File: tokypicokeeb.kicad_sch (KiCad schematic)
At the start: 119 parts, among them SW1 SW_Push, U1 PicoW

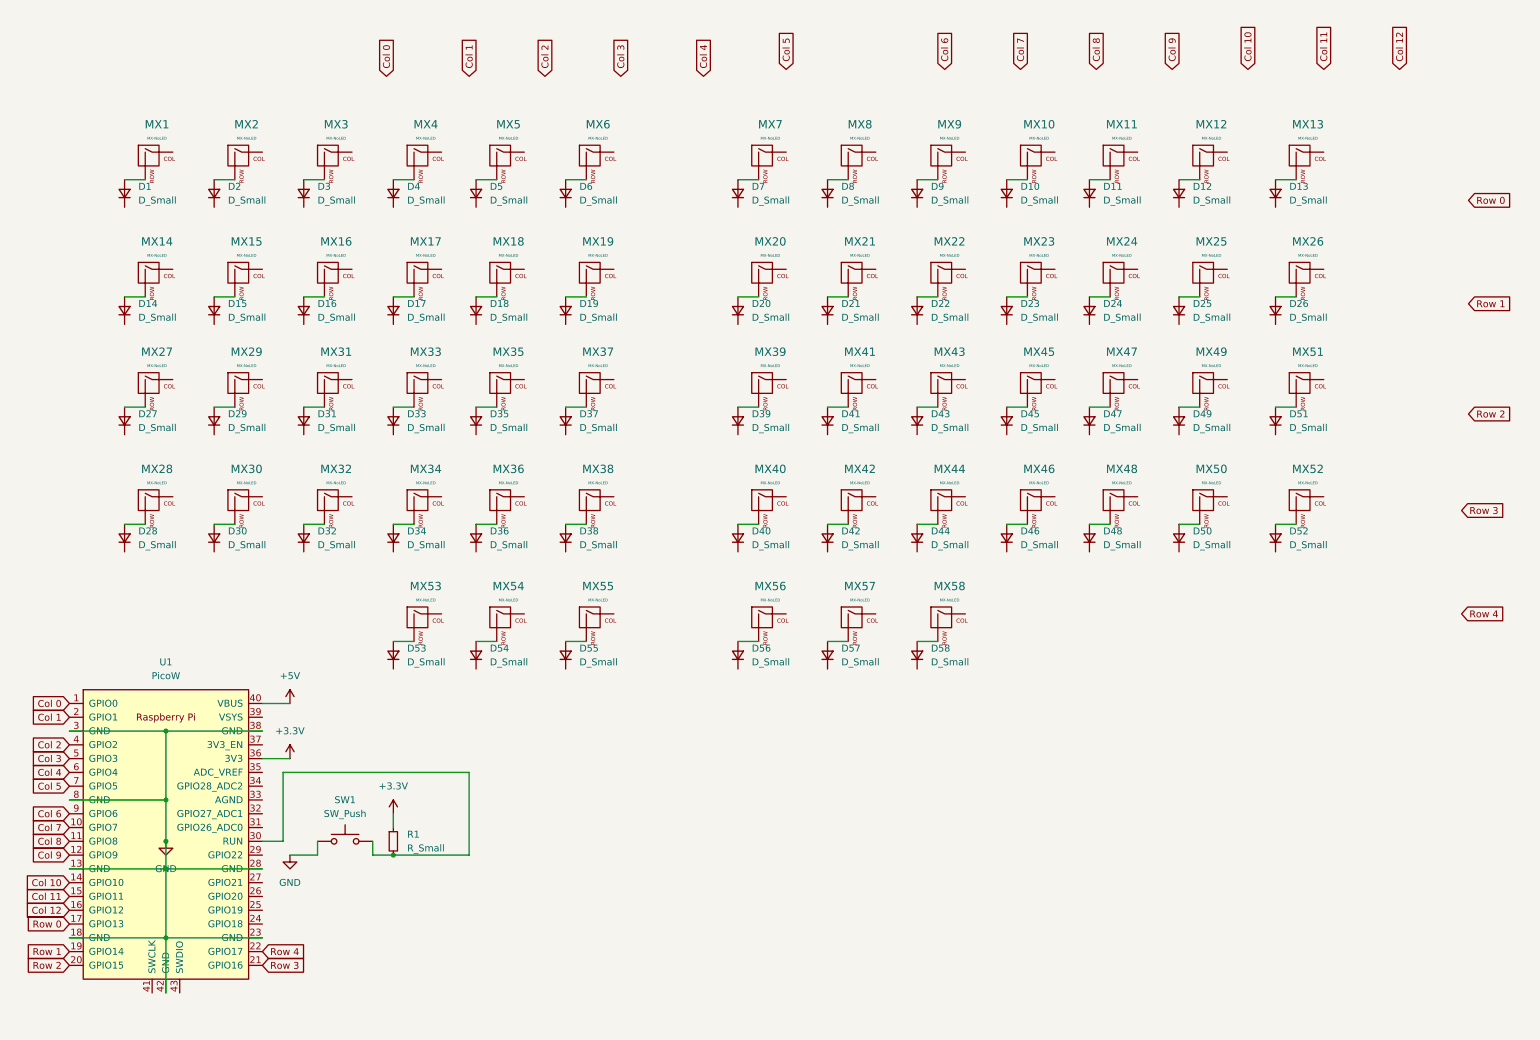
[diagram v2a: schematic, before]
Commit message: pcb stage 1
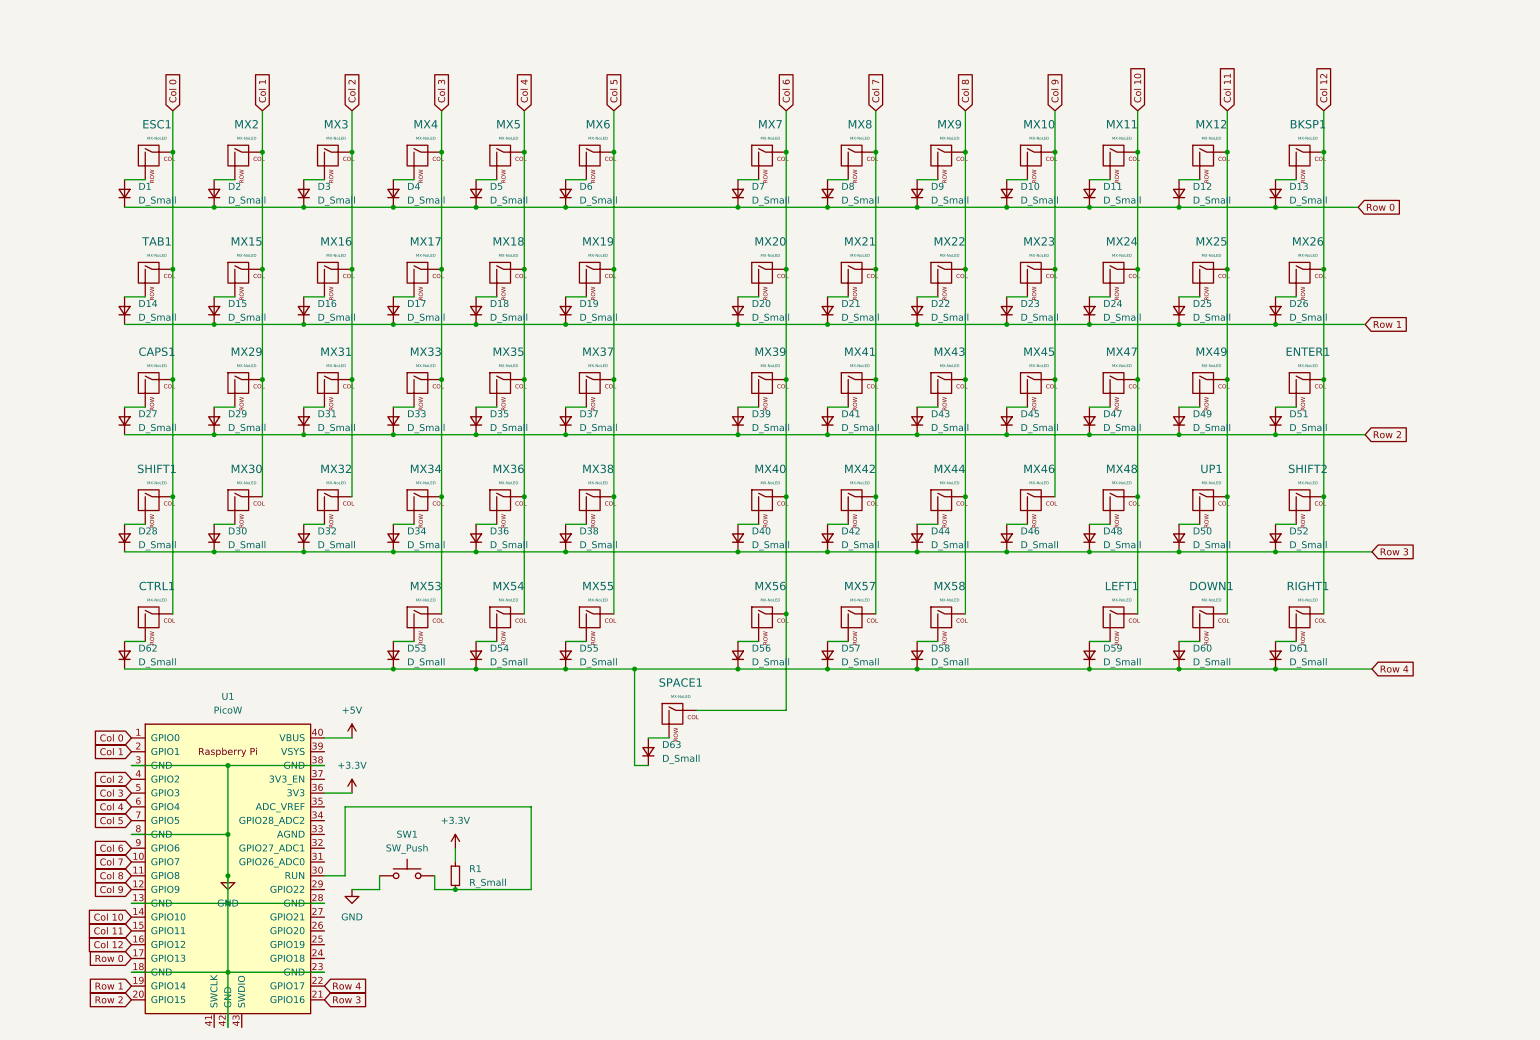
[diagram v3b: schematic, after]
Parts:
- added CTRL1: MX-NoLED, MX_Alps_Hybrid:MX-1.25U-NoLED, symbol MX_Alps_Hybrid:MX-NoLED
- added D59, D60, D61, D62, D63: D_Small, random-keyboard-parts:D_SOD-123-Pretty, symbol Device:D_Small
- added DOWN1, LEFT1, RIGHT1: MX-NoLED, MX_Alps_Hybrid:MX-1U-NoLED, symbol MX_Alps_Hybrid:MX-NoLED
- added SPACE1: MX-NoLED, MX_Alps_Hybrid:MX-6.25U-NoLED, symbol MX_Alps_Hybrid:MX-NoLED
- BKSP1: renamed from MX13; footprint (none) -> MX_Alps_Hybrid:MX-2U-NoLED
- CAPS1: renamed from MX27; footprint (none) -> MX_Alps_Hybrid:MX-1.75U-NoLED
- D1, D10, D11, D12, D13, D14, D15, D16, D17, D18, D19, D2, D20, D21, D22, D23, D24, D25, D26, D27, D28, D29, D3, D30, D31, D32, D33, D34, D35, D36, D37, D38, D39, D4, D40, D41, D42, D43, D44, D45, D46, D47, D48, D49, D5, D50, D51, D52, D53, D54, D55, D56, D57, D58, D6, D7, D8, D9: footprint (none) -> random-keyboard-parts:D_SOD-123-Pretty
- ENTER1: renamed from MX51; footprint (none) -> MX_Alps_Hybrid:MX-2.5U-NoLED
- ESC1: renamed from MX1; footprint (none) -> MX_Alps_Hybrid:MX-1U-NoLED
- MX10, MX11, MX12, MX15, MX16, MX17, MX18, MX19, MX2, MX20, MX21, MX22, MX23, MX24, MX25, MX26, MX29, MX3, MX30, MX31, MX32, MX33, MX34, MX35, MX36, MX37, MX38, MX39, MX4, MX40, MX41, MX42, MX43, MX44, MX45, MX46, MX47, MX48, MX49, MX5, MX53, MX54, MX55, MX56, MX57, MX58, MX6, MX7, MX8, MX9: footprint (none) -> MX_Alps_Hybrid:MX-1U-NoLED
- R1: footprint (none) -> Resistor_SMD:R_0805_2012Metric
- SHIFT1: renamed from MX28; footprint (none) -> MX_Alps_Hybrid:MX-2.25U-NoLED
- SHIFT2: renamed from MX52; footprint (none) -> MX_Alps_Hybrid:MX-2.75U-NoLED
- SW1: footprint (none) -> random-keyboard-parts:SKQG-1155865
- TAB1: renamed from MX14; footprint (none) -> MX_Alps_Hybrid:MX-1.5U-NoLED
- U1: footprint RPiPicoW:RPi_PicoW_SMD_TH -> pico_w:RPi_PicoW_SMD_TH
- UP1: renamed from MX50; footprint (none) -> MX_Alps_Hybrid:MX-1U-NoLED
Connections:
- net Col 0: now also CAPS1.1 (COL), ESC1.1 (COL), SHIFT1.1 (COL), TAB1.1 (COL), CTRL1.1 (COL)
- net Col 1: now also MX15.1 (COL), MX2.1 (COL), MX29.1 (COL), MX30.1 (COL)
- net Col 10: now also MX11.1 (COL), MX24.1 (COL), MX47.1 (COL), MX48.1 (COL), LEFT1.1 (COL)
- net Col 11: now also MX12.1 (COL), MX25.1 (COL), MX49.1 (COL), UP1.1 (COL), DOWN1.1 (COL)
- net Col 12: now also BKSP1.1 (COL), ENTER1.1 (COL), MX26.1 (COL), SHIFT2.1 (COL), RIGHT1.1 (COL)
- net Col 2: now also MX16.1 (COL), MX3.1 (COL), MX31.1 (COL), MX32.1 (COL)
- net Col 3: now also MX17.1 (COL), MX33.1 (COL), MX34.1 (COL), MX4.1 (COL), MX53.1 (COL)
- net Col 4: now also MX18.1 (COL), MX35.1 (COL), MX36.1 (COL), MX5.1 (COL), MX54.1 (COL)
- net Col 5: now also MX19.1 (COL), MX37.1 (COL), MX38.1 (COL), MX55.1 (COL), MX6.1 (COL)
- net Col 6: now also MX20.1 (COL), MX39.1 (COL), MX40.1 (COL), MX56.1 (COL), MX7.1 (COL), SPACE1.1 (COL)
- net Col 7: now also MX21.1 (COL), MX41.1 (COL), MX42.1 (COL), MX57.1 (COL), MX8.1 (COL)
- net Col 8: now also MX22.1 (COL), MX43.1 (COL), MX44.1 (COL), MX58.1 (COL), MX9.1 (COL)
- net Col 9: now also MX10.1 (COL), MX23.1 (COL), MX45.1 (COL), MX46.1 (COL)
- net Row 0: now also D1.1 (K), D10.1 (K), D11.1 (K), D12.1 (K), D13.1 (K), D2.1 (K), D3.1 (K), D4.1 (K), D5.1 (K), D6.1 (K), D7.1 (K), D8.1 (K), D9.1 (K)
- net Row 1: now also D14.1 (K), D15.1 (K), D16.1 (K), D17.1 (K), D18.1 (K), D19.1 (K), D20.1 (K), D21.1 (K), D22.1 (K), D23.1 (K), D24.1 (K), D25.1 (K), D26.1 (K)
- net Row 2: now also D27.1 (K), D29.1 (K), D31.1 (K), D33.1 (K), D35.1 (K), D37.1 (K), D39.1 (K), D41.1 (K), D43.1 (K), D45.1 (K), D47.1 (K), D49.1 (K), D51.1 (K)
- net Row 3: now also D28.1 (K), D30.1 (K), D32.1 (K), D34.1 (K), D36.1 (K), D38.1 (K), D40.1 (K), D42.1 (K), D44.1 (K), D46.1 (K), D48.1 (K), D50.1 (K), D52.1 (K)
- net Row 4: now also D53.1 (K), D54.1 (K), D55.1 (K), D56.1 (K), D57.1 (K), D58.1 (K), D59.1 (K), D60.1 (K), D61.1 (K), D62.1 (K), D63.1 (K)
- new net: D60.2 (A), DOWN1.2 (ROW)
- new net: D61.2 (A), RIGHT1.2 (ROW)
- new net: D63.2 (A), SPACE1.2 (ROW)
- new net: D59.2 (A), LEFT1.2 (ROW)
- new net: CTRL1.2 (ROW), D62.2 (A)
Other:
- moved on the sheet: R1, SW1, U1
